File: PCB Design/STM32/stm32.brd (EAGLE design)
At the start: 71.1 x 84.3 mm, 68 parts, among them IC1 NCP1117ST50T3G, Q1 ABM3B-8.000MHZ-10-1UT, T5 BC847, T6 BC847, T7 BC847, T8 BC847, U1 STM32F103RET6, U2 MCP1700T-3302E/TT, U3 MCP1700T-3302E/TT, U4 MPU-6050, U5 TB6612FNG, X1 22-23-2031

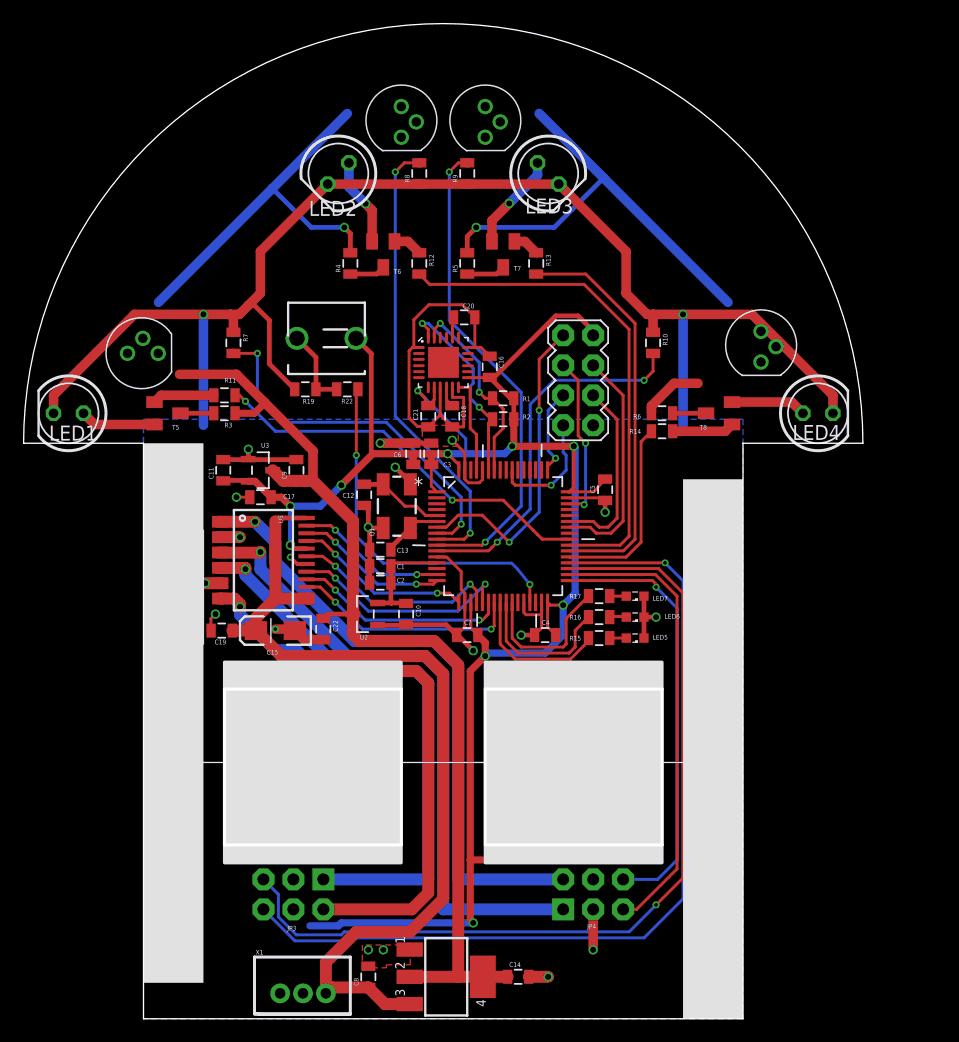
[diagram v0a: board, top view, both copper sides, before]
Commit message: save
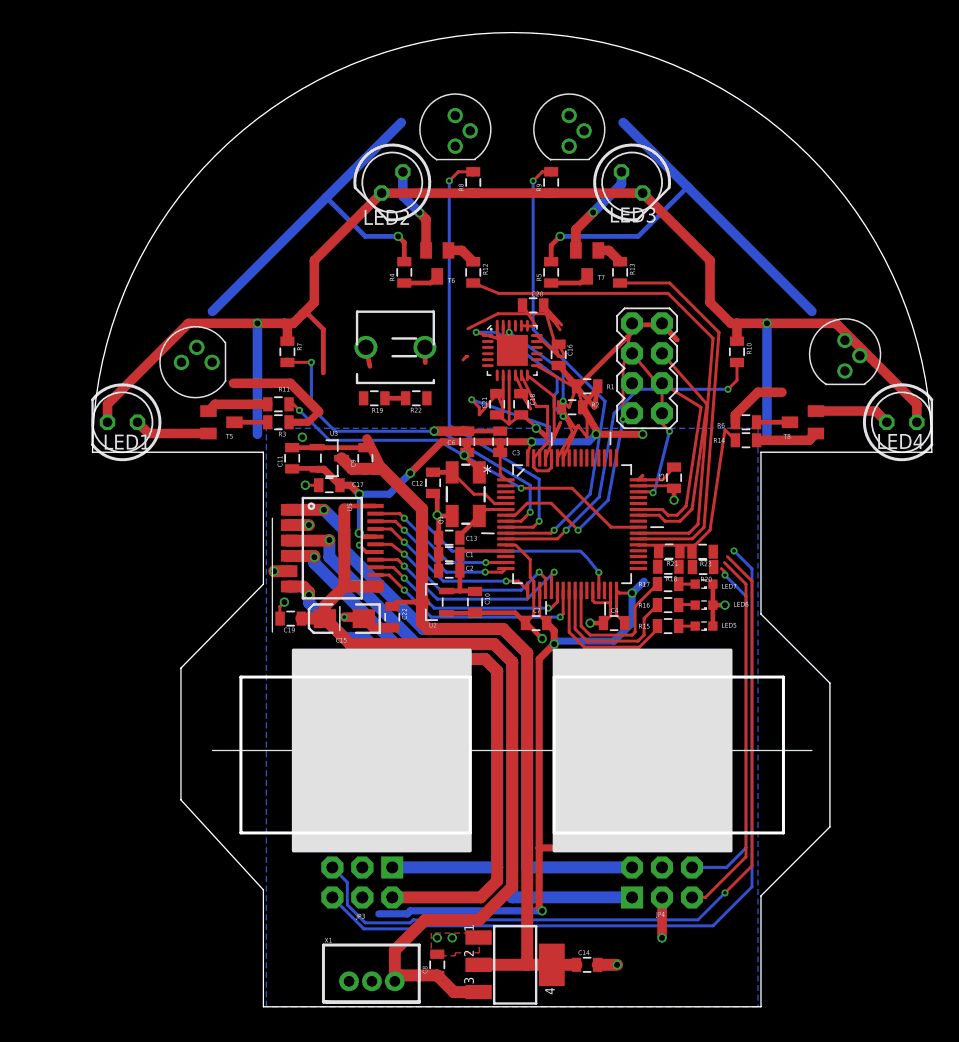
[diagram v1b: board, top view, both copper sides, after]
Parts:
- added R18, R20, R21, R23: (no value), SparkFun-Resistors:0805
- moved R1 7.18 mm to (50.0, 56.4)
- moved U$5 7.15 mm to (71.9, 59.2)
- moved LED3 7.15 mm to (53.8, 73.7)
- moved R10 7.15 mm to (62.7, 59.3)
- moved R13 7.15 mm to (52.8, 66.0)
- moved R14 7.15 mm to (63.5, 51.8)
- moved R5 7.15 mm to (47.0, 66.0)
- moved R6 7.15 mm to (63.5, 53.3)
- moved R9 7.15 mm to (47.0, 73.7)
- moved U$4 7.15 mm to (48.5, 78.2)
- moved LED4 7.15 mm to (76.7, 53.3)
- moved T8 7.15 mm to (68.3, 53.3)
- moved T7 7.15 mm to (50.0, 66.8)
- moved LED7 5.93 mm to (59.9, 39.6)
- moved C10 5.93 mm to (40.5, 38.1)
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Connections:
- new net N$20: R18.2, U1.33
- new net N$21: R20.2, U1.34
- new net N$29: R21.2, U1.35
- new net N$30: R23.2, U1.36
- net M1CA: now also R18.1; no longer U1.33
- net M1CB: now also R20.1; no longer U1.34
- net M2CA: now also R23.1; no longer U1.36
- net M2CB: now also R21.1; no longer U1.35
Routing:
- net BUTTON1: track 30.5 -> 18.0 mm, vias 2 -> 1
- net JTAG-TDO: track 10.2 -> 0.00 mm, vias 1 -> 0
- net GND: track 233.1 -> 241.9 mm
- net M2CA: track 75.3 -> 67.2 mm
- net VCC: track 172.1 -> 164.4 mm
- net M2CB: track 75.2 -> 67.7 mm
- net JTAG-TCK: track 7.40 -> 0.00 mm, vias 1 -> 0
- net M1CB: track 39.0 -> 31.7 mm
- net M1CA: track 36.8 -> 29.8 mm
- net I2C1_SDA: track 17.0 -> 23.2 mm
- net 5V: track 161.7 -> 156.3 mm
- net I2C1_SCL: track 16.7 -> 21.3 mm
- net N$31: track 6.74 -> 3.40 mm
- net N$10: track 1.75 -> 4.63 mm
- net INT: track 8.22 -> 11.0 mm
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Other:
- board size 71.1 x 84.3 mm -> 71.1 x 82.5 mm
